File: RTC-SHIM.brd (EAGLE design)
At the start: 25.4 x 50.8 mm, 15 parts, among them IC1 DS3231/SO

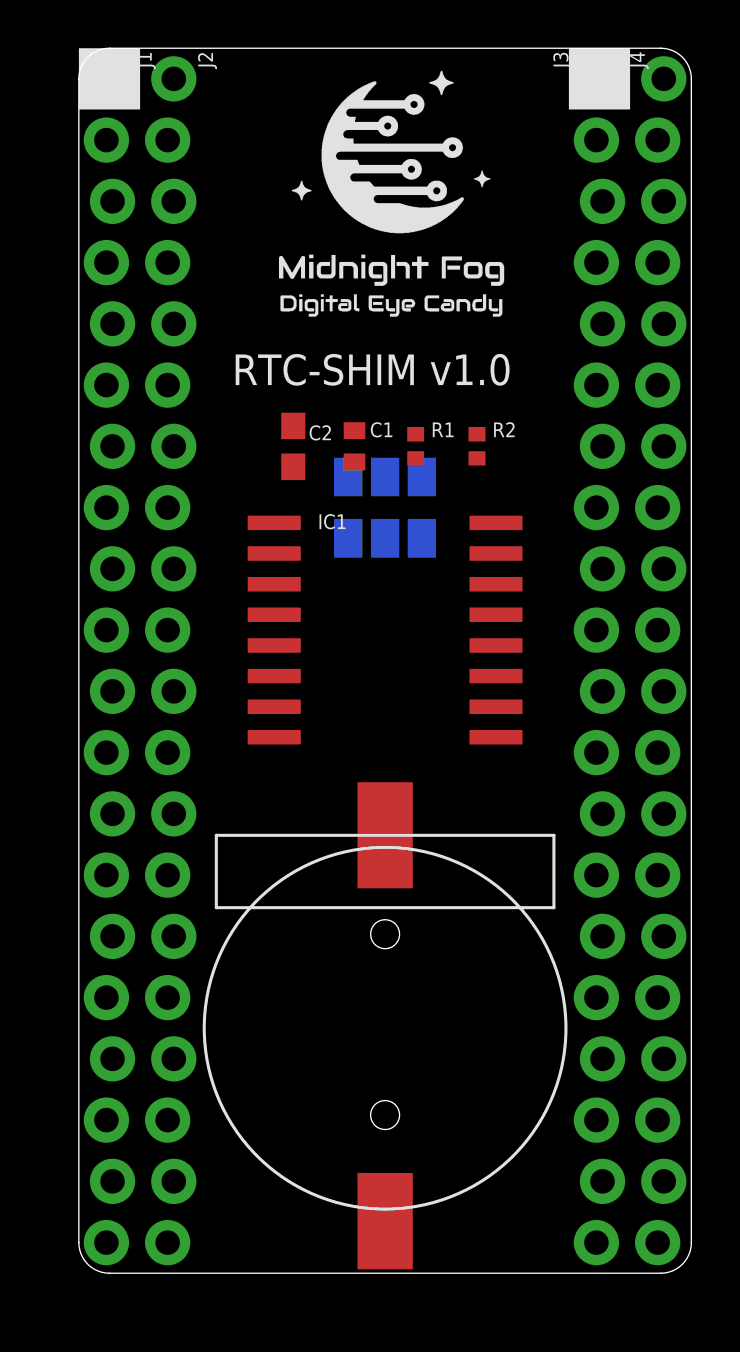
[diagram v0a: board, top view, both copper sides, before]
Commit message: Moved stuff around a little bit.
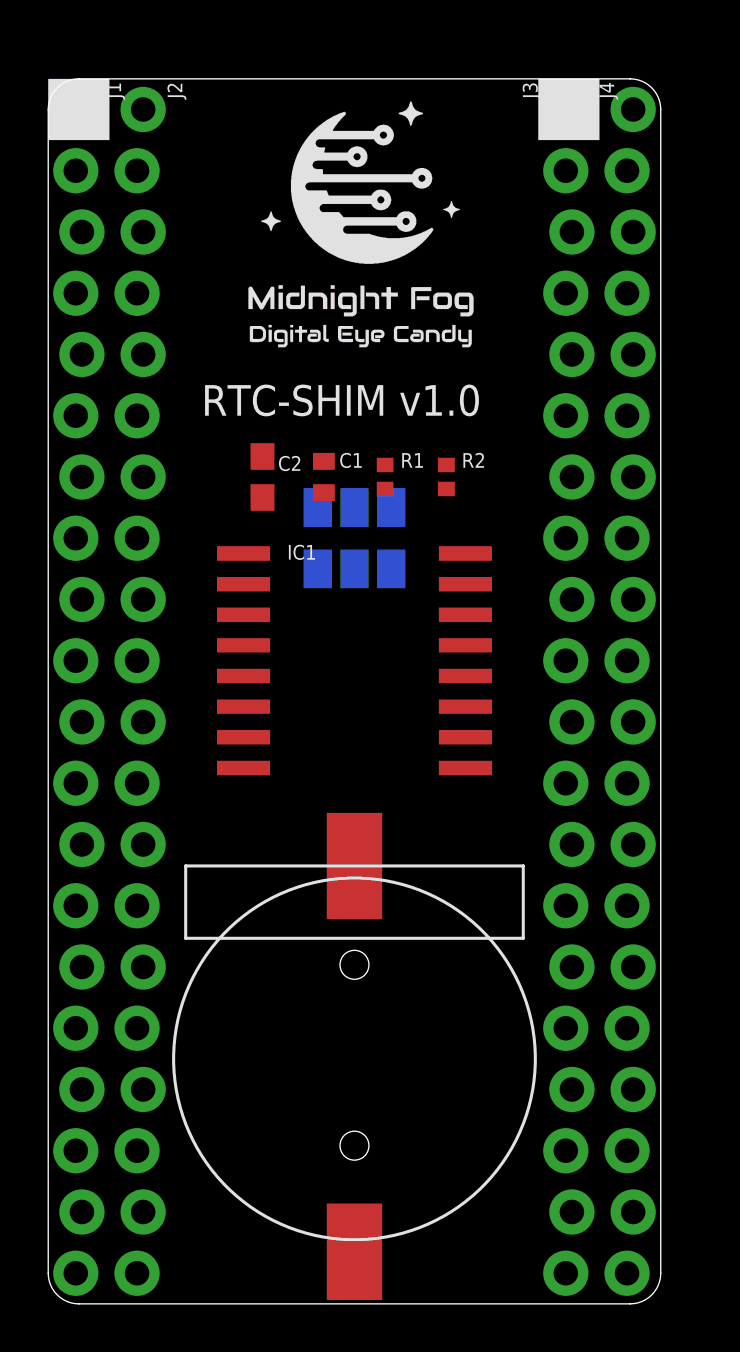
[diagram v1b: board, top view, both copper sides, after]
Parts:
- moved LOGO1 1.80 mm to (7.62, 39.4)
- moved C1 1.80 mm to (11.4, 34.3)
- moved C2 1.80 mm to (8.89, 34.3)
- moved LOGO3 1.80 mm to (17.8, 39.4)
- moved R1 1.80 mm to (14.0, 34.3)
- moved R2 1.80 mm to (16.5, 34.3)
- moved BAT1 1.80 mm to (12.7, 10.2)
- moved IC1 1.80 mm to (12.7, 26.7)
- moved SJ2 1.80 mm to (12.7, 30.5)
- moved LOGO2 1.80 mm to (-0.25, -5.71)
- moved SJ1 1.80 mm to (12.7, 33.0)
- moved J1 1.80 mm to (1.27, 49.5)
- moved J2 1.80 mm to (3.81, 49.5)
- moved J3 1.80 mm to (21.6, 49.5)
- moved J4 1.80 mm to (24.1, 49.5)
